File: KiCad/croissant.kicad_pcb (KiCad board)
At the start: 2 copper layers, 149.8 x 90.3 mm, 53 parts, among them J1 USB_C_Receptacle_PowerOnly_6P, Q1 NMOS, SW1 SW_SPDT, U1 NE556, U2 TL064

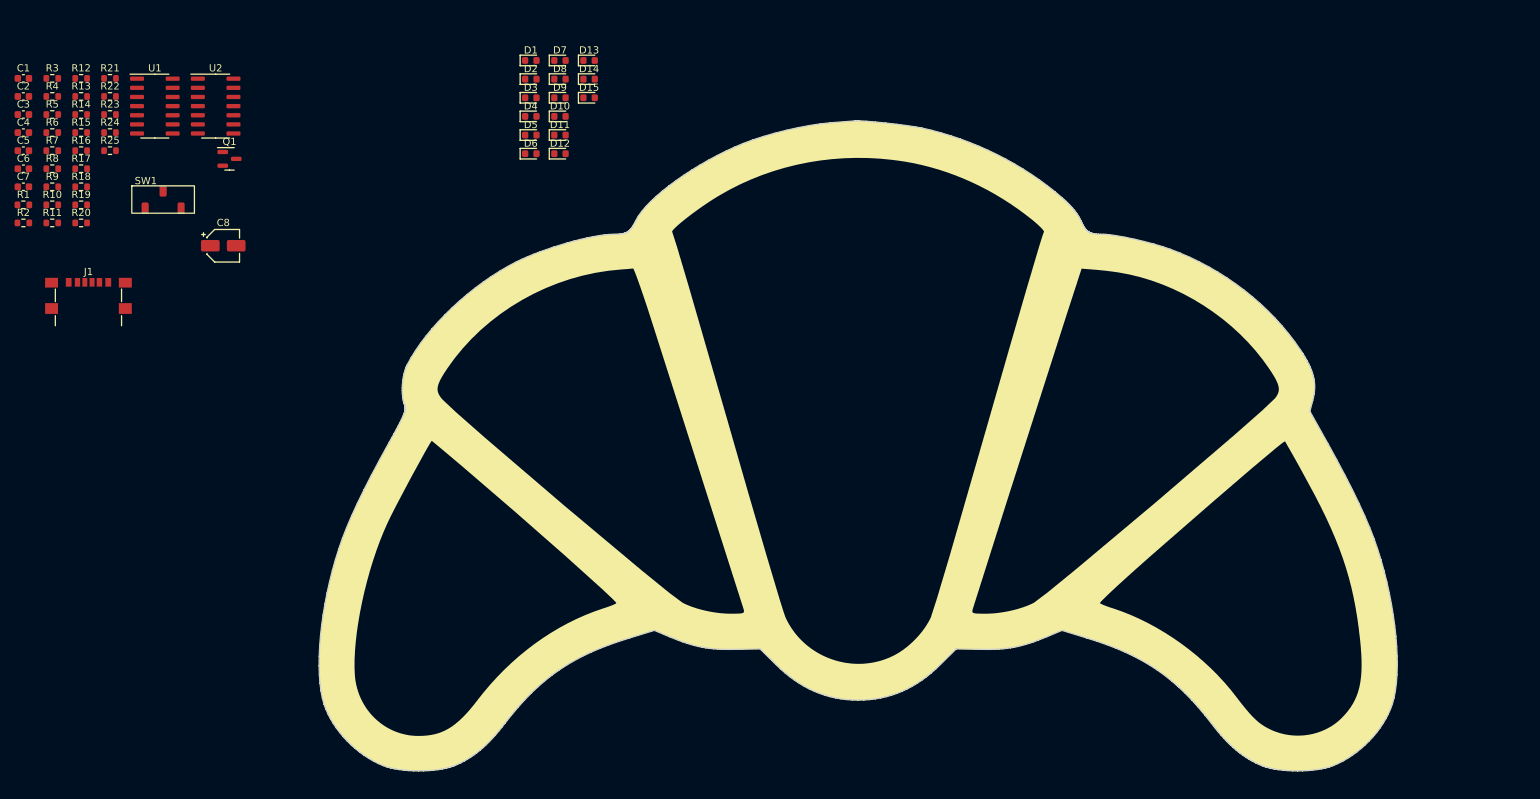
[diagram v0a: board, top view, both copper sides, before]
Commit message: Advance routing
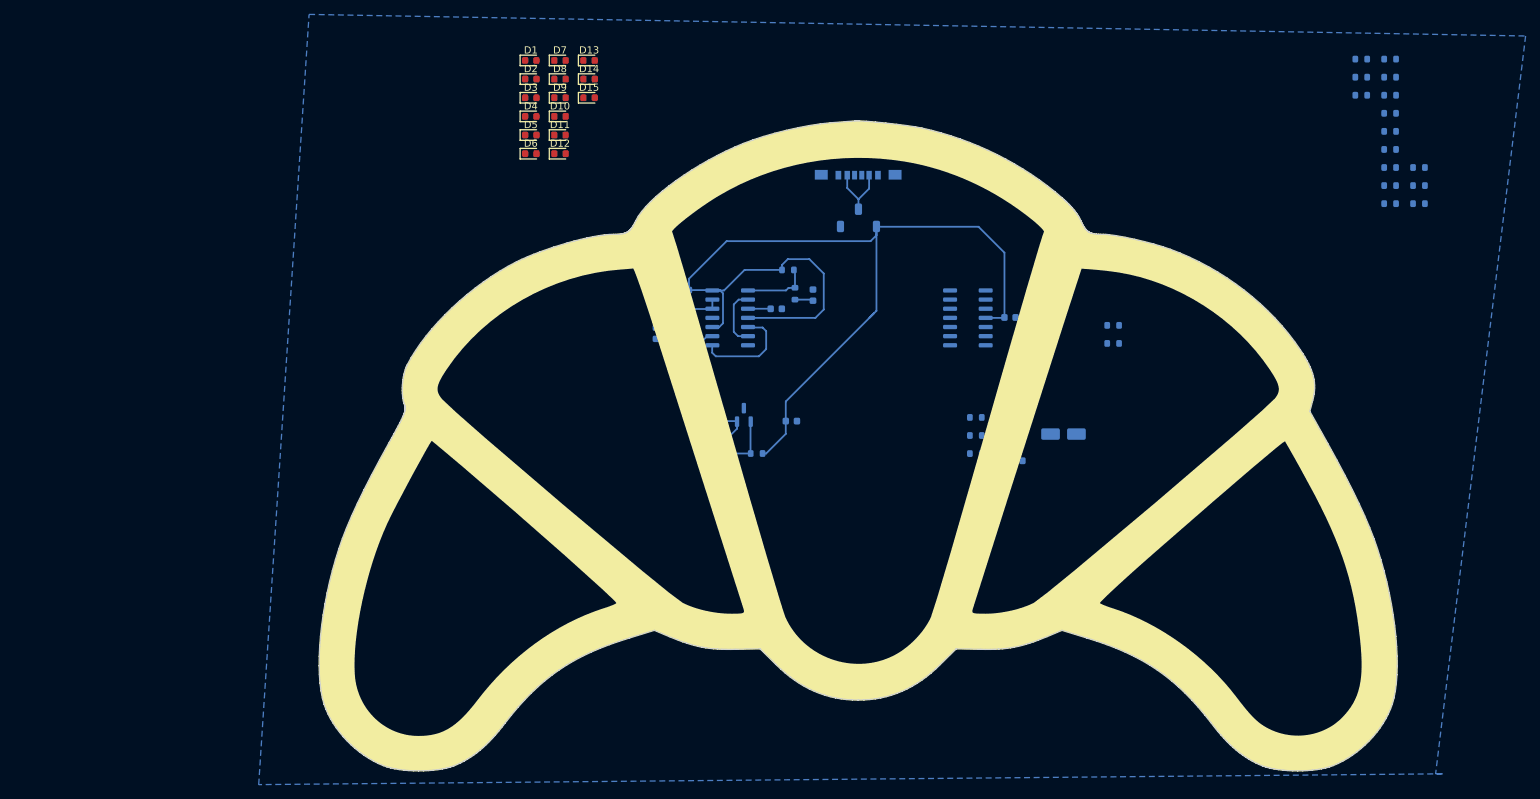
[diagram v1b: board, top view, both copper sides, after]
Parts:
- C1: value C -> 0.1u; moved to B.Cu
- C2, C3, C4, C5, C6, C7, C8, J1, Q1, R1, R10, R11, R12, R13, R14, R15, R16, R17, R18, R19, R2, R20, R21, R22, R23, R24, R25, R3, R4, R5, R6, R7, R8, R9, SW1, U1, U2: moved to B.Cu
- moved R10 189.9 mm to (222.7, 55.3), turned to 180 degrees
- moved R11 189.9 mm to (222.7, 57.8), turned to 180 degrees
- moved R9 189.9 mm to (222.7, 52.8), turned to 180 degrees
- moved R12 181.9 mm to (218.7, 37.7), turned to 180 degrees
- moved R13 181.9 mm to (218.7, 40.2), turned to 180 degrees
- moved R14 181.9 mm to (218.7, 42.7), turned to 180 degrees
- moved R15 181.9 mm to (218.7, 45.2), turned to 180 degrees
- moved R16 181.9 mm to (218.7, 47.8), turned to 180 degrees
- moved R17 181.9 mm to (218.7, 50.3), turned to 180 degrees
- moved R18 181.9 mm to (218.7, 52.8), turned to 180 degrees
- moved R19 181.9 mm to (218.7, 55.3), turned to 180 degrees
- moved R20 181.9 mm to (218.7, 57.8), turned to 180 degrees
- moved R21 173.8 mm to (214.7, 37.7), turned to 180 degrees
- moved R22 173.8 mm to (214.7, 40.2), turned to 180 degrees
- moved R23 173.8 mm to (214.7, 42.7), turned to 180 degrees
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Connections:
- C4 pad 1: +5V -> GND
- C4 pad 2: GND -> Net-(U1A-CV)
- U1 pad 3: unconnected-(U1A-CV-Pad3) -> Net-(U1A-CV)
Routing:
- net +5V: track 0.00 -> 152.0 mm
- net Net-(Q1-G): track 0.00 -> 21.9 mm
- net /PulseOut: track 0.00 -> 14.4 mm
- net Net-(U1B-DIS): track 0.00 -> 11.7 mm
- net Net-(U1A-THR): track 0.00 -> 10.8 mm
- net Net-(SW1-B): track 0.00 -> 9.33 mm
- net Net-(U1A-DIS): track 0.00 -> 9.13 mm
- net /PWMOut: track 0.00 -> 7.02 mm
- net Net-(U1A-CV): track 0.00 -> 3.15 mm
- added copper zone on B.Cu, net GND
